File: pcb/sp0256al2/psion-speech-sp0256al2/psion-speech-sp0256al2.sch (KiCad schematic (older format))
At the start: 29 parts, among them J1 Connector_USB_B_Micro, J3 Conn_02x08_Odd_Even, U1 SP0256AL2, U2 74LS368, U3 PAM8302AAD, U4 4011, Y1 3.2768MHz

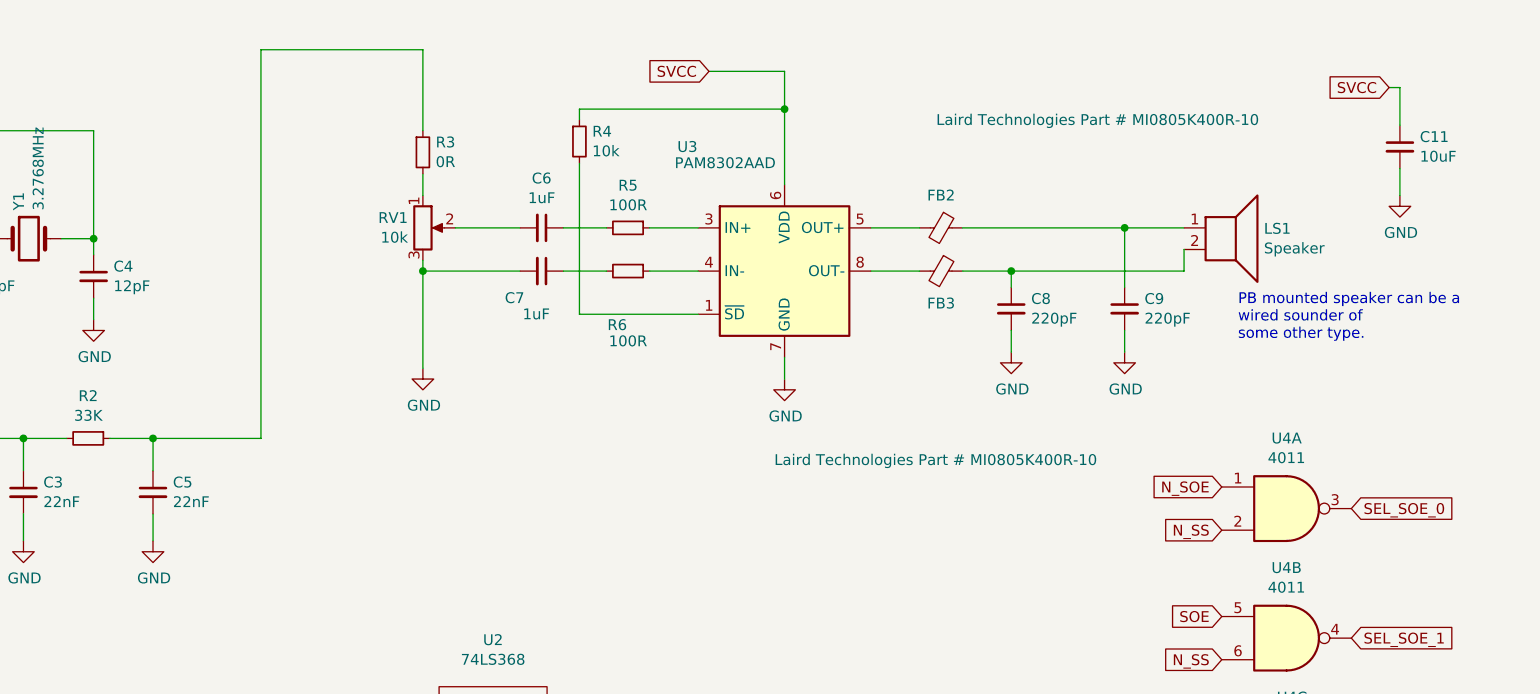
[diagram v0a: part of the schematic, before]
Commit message: Updates
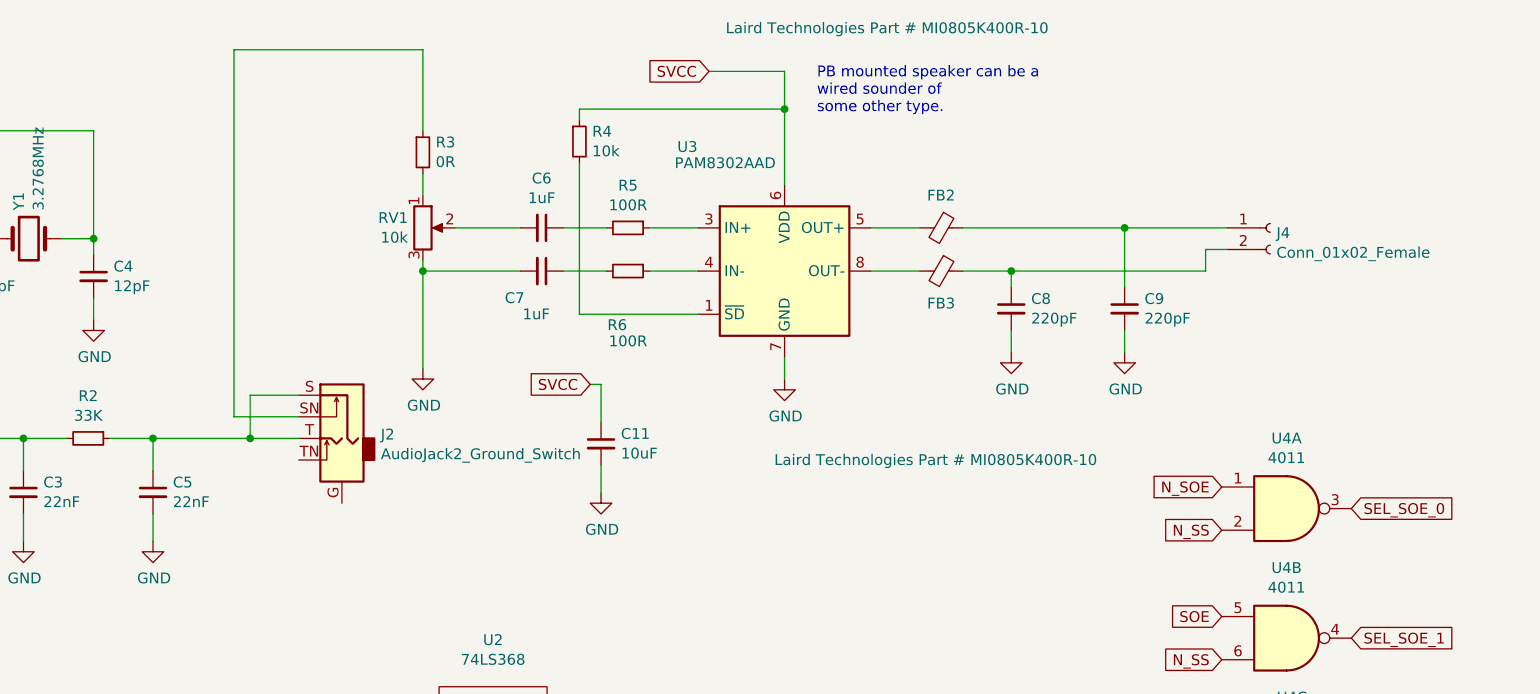
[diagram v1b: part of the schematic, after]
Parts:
- removed LS1: Speaker, symbol Device:Speaker
- added J2: AudioJack2_Ground_Switch, symbol Connector:AudioJack2_Ground_Switch
- added J4: Conn_01x02_Female, Connector_PinHeader_2.54mm:PinHeader_1x02_P2.54mm_Vertical, symbol Connector:Conn_01x02_Female
- Y1: footprint (none) -> psion_org_2:crystal_um4s
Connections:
- net at C9.1, FB2.1: now also J4.1 (Pin_1)
- net at C8.1, FB3.1: now also J4.2 (Pin_2)
- net at C5.1, R2.1: now also J2.S, J2.T; no longer R3.1
- new net: J2.SN, R3.1
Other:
- moved on the sheet: C11
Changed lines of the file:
@@
 F 0 "Y1" V 4254 1756 50  0000 L CNN
 F 1 "3.2768MHz" V 4345 1756 50  0000 L CNN
-F 2 "" H 4300 1625 50  0001 C CNN
+F 2 "psion_org_2:crystal_um4s" H 4300 1625 50  0001 C CNN
 F 3 "~" H 4300 1625 50  0001 C CNN
 	1    4300 1625
@@
 AR Path="/63427936" Ref="FB2"  Part="1"
 F 0 "FB2" V 8375 1575 50  0000 C CNN
-F 1 "Laird Technologies Part # MI0805K400R-10" V 8025 2300 50  0000 C CNN
+F 1 "Laird Technologies Part # MI0805K400R-10" V 7600 1325 50  0000 C CNN
 F 2 "Capacitor_SMD:C_0805_2012Metric" V 8455 1575 50  0001 C CNN
 F 3 "~" H 8525 1575 50  0001 C CNN
@@
 Wire Wire Line
 	8850 1775 8850 1850
-Wire Wire Line
-	9650 1575 9375 1575
 Connection ~ 9375 1575
-Wire Wire Line
-	9650 1675 9650 1775
-Wire Wire Line
-	9650 1775 8850 1775
 Wire Wire Line
 	9375 1575 9375 1850
@@
 Wire Wire Line
 	6125 1325 6125 1425
-Wire Wire Line
-	4875 2550 5375 2550
-Wire Wire Line
-	5375 2550 5375 750
-Wire Wire Line
-	5375 750  6125 750
 Wire Wire Line
 	6125 750  6125 1125
@@
 L Device:C_Small C11
 U 1 1 6348419A
-P 10650 1200
-F 0 "C11" H 10742 1246 50  0000 L CNN
-F 1 "10uF" H 10742 1155 50  0000 L CNN
-F 2 "Capacitor_SMD:C_1210_3225Metric_Pad1.33x2.70mm_HandSolder" H 10650 1200 50  0001 C CNN
-F 3 "~" H 10650 1200 50  0001 C CNN
-	1    10650 1200
+P 6950 2575
+F 0 "C11" H 7042 2621 50  0000 L CNN
+F 1 "10uF" H 7042 2530 50  0000 L CNN
+F 2 "Capacitor_SMD:C_1210_3225Metric_Pad1.33x2.70mm_HandSolder" H 6950 2575 50  0001 C CNN
+F 3 "~" H 6950 2575 50  0001 C CNN
+	1    6950 2575
 	1    0    0    -1
 $EndComp
@@
 L power:GND #PWR014
 U 1 1 63484BC1
-P 10650 1425
-F 0 "#PWR014" H 10650 1175 50  0001 C CNN
-F 1 "GND" H 10655 1252 50  0000 C CNN
-F 2 "" H 10650 1425 50  0001 C CNN
-F 3 "" H 10650 1425 50  0001 C CNN
-	1    10650 1425
-	1    0    0    -1
-$EndComp
-Text GLabel 10600 925  0    50   Input ~ 0
+P 6950 2800
+F 0 "#PWR014" H 6950 2550 50  0001 C CNN
+F 1 "GND" H 6955 2627 50  0000 C CNN
+F 2 "" H 6950 2800 50  0001 C CNN
+F 3 "" H 6950 2800 50  0001 C CNN
+	1    6950 2800
+	1    0    0    -1
+$EndComp
+Text GLabel 6900 2300 0    50   Input ~ 0
 SVCC
 Wire Wire Line
-	10600 925  10650 925
-Wire Wire Line
-	10650 925  10650 1100
-Wire Wire Line
-	10650 1300 10650 1425
+	6900 2300 6950 2300
+Wire Wire Line
+	6950 2300 6950 2475
+Wire Wire Line
+	6950 2675 6950 2800
 Text GLabel 2050 4150 2    50   Input ~ 0
 SD1
@@
 	1    0    0    -1
 $EndComp
-$Comp
-L Device:Speaker LS1
-U 1 1 63412366
-P 9850 1575
-F 0 "LS1" H 10020 1571 50  0000 L CNN
-F 1 "Speaker" H 10020 1480 50  0000 L CNN
-F 2 "" H 9850 1375 50  0001 C CNN
-F 3 "~" H 9840 1525 50  0001 C CNN
-	1    9850 1575
-	1    0    0    -1
-$EndComp
-Text Notes 9900 2100 0    50   ~ 0
+Text Notes 7950 1050 0    50   ~ 0
 PB mounted speaker can be a\nwired sounder of\nsome other type.
+$Comp
+L Connector:AudioJack2_Ground_Switch J2
+U 1 1 6343E58B
+P 5750 2550
+F 0 "J2" H 5570 2568 50  0000 R CNN
+F 1 "AudioJack2_Ground_Switch" H 5570 2477 50  0000 R CNN
+F 2 "" H 5750 2750 50  0001 C CNN
+F 3 "~" H 5750 2750 50  0001 C CNN
+	1    5750 2550
+	-1   0    0    -1
+$EndComp
+Wire Wire Line
+	9375 1575 9850 1575
+Wire Wire Line
+	9850 1675 9750 1675
+Wire Wire Line
+	9750 1675 9750 1775
+Wire Wire Line
+	8850 1775 9750 1775
+Wire Wire Line
+	4875 2550 5325 2550
+Wire Wire Line
+	5325 2550 5325 2350
+Wire Wire Line
+	5325 2350 5550 2350
+Connection ~ 5325 2550
+Wire Wire Line
+	5325 2550 5550 2550
+Wire Wire Line
+	5250 2450 5250 750
+Wire Wire Line
+	5250 750  6125 750
+Wire Wire Line
+	5250 2450 5550 2450
+$Comp
+L Connector:Conn_01x02_Female J4
+U 1 1 634738A3
+P 10050 1575
+F 0 "J4" H 10078 1551 50  0000 L CNN
+F 1 "Conn_01x02_Female" H 10078 1460 50  0000 L CNN
+F 2 "Connector_PinHeader_2.54mm:PinHeader_1x02_P2.54mm_Vertical" H 10050 1575 50  0001 C CNN
+F 3 "~" H 10050 1575 50  0001 C CNN
+	1    10050 1575
+	1    0    0    -1
+$EndComp
 $EndSCHEMATC
